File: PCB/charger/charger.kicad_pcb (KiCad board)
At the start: 2 copper layers, 26.9 x 17 mm, 18 parts, among them J1 Conn_01x02_Socket, J2 USB_C_Receptacle, J3 Conn_01x02_Socket, J4 Conn_01x02_Socket, J5 Conn_01x02_Socket, Q2 BSS83P, U1 MCP73831T-2ACI/OT

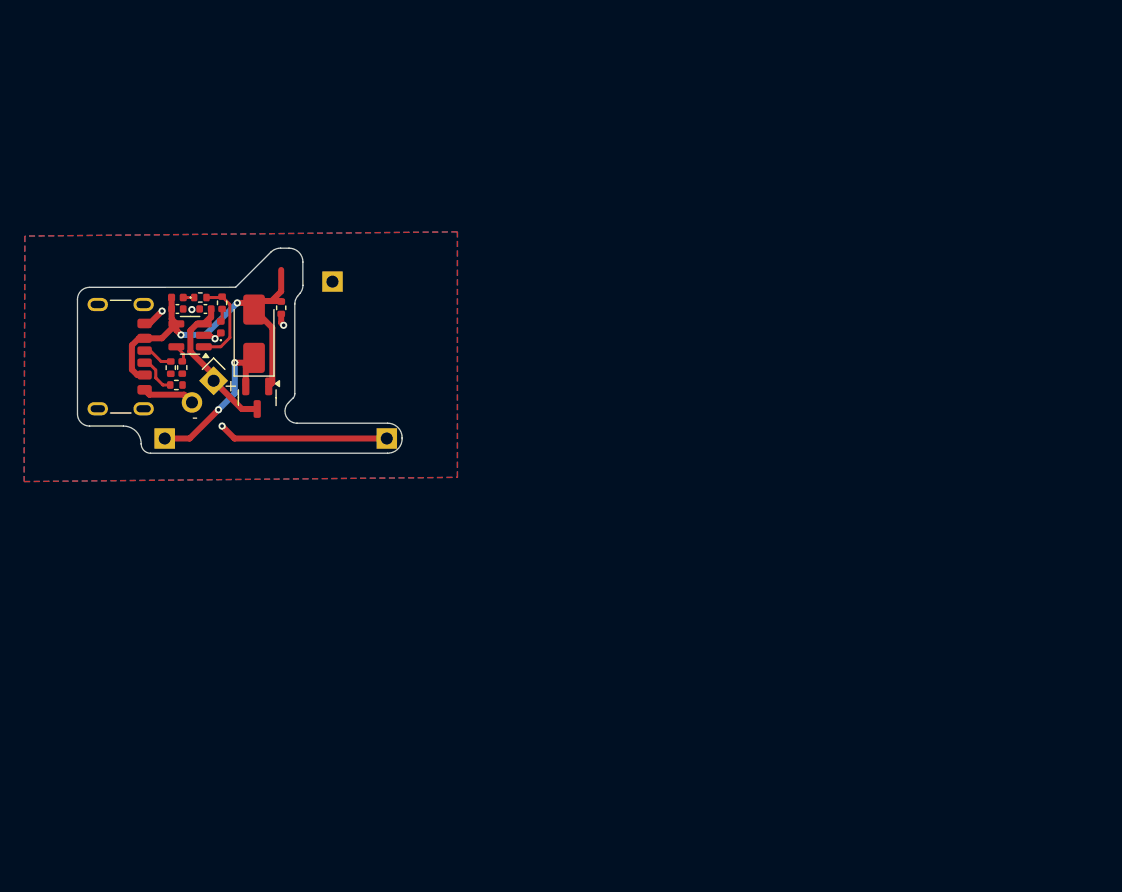
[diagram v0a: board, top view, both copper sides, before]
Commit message: idk
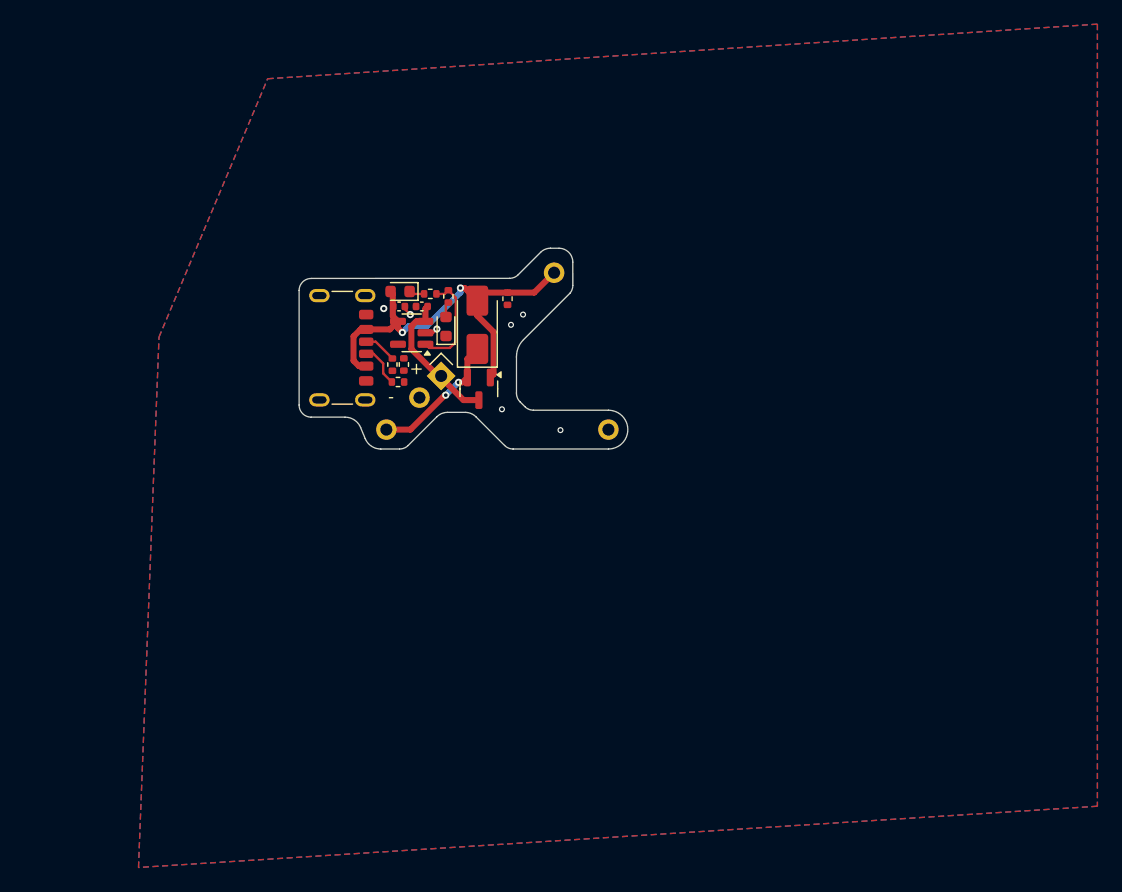
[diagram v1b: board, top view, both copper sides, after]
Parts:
- D1, D2: footprint LED_SMD:LED_0402_1005Metric -> LED_SMD:LED_0603_1608Metric
- J3, J4, J5: moved to B.Cu
- moved R2 19.1 mm to (73.7, 73.4)
- moved J1 18.9 mm to (74.6, 80.2)
- moved R6 18.8 mm to (80.1, 73.8)
- moved R3 18.8 mm to (75.2, 73.6)
- moved D2 18.7 mm to (75.0, 76.1)
- moved D3 18.5 mm to (77.6, 76.0)
- moved D1 18.5 mm to (71.2, 73.2)
- moved J3 18.4 mm to (70.1, 84.6), turned to 180 degrees
- moved J2 18.4 mm to (65.3, 77.9)
- moved J4 18.4 mm to (88.5, 84.6), turned to 180 degrees
- moved J5 18.4 mm to (84.0, 71.6), turned to 180 degrees
- moved Q2 18.4 mm to (77.7, 81.3)
- moved R1 18.4 mm to (71.0, 80.7)
- moved R5 18.4 mm to (71.5, 79.2)
- moved R4 18.4 mm to (70.6, 79.3)
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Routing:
- net GND: track 23.2 -> 2.32 mm, vias 5 -> 7
- net VOUT: track 14.6 -> 11.2 mm
- net 5V: track 31.1 -> 34.0 mm
- net Net-(U1-PROG): track 1.53 -> 0.00 mm
- net Net-(U1-STAT): track 7.46 -> 8.50 mm
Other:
- board size 26.9 x 17 mm -> 27.2 x 16.6 mm
